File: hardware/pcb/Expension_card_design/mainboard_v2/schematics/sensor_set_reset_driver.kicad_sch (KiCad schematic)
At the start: 9 parts, among them U3 OPA2197xD

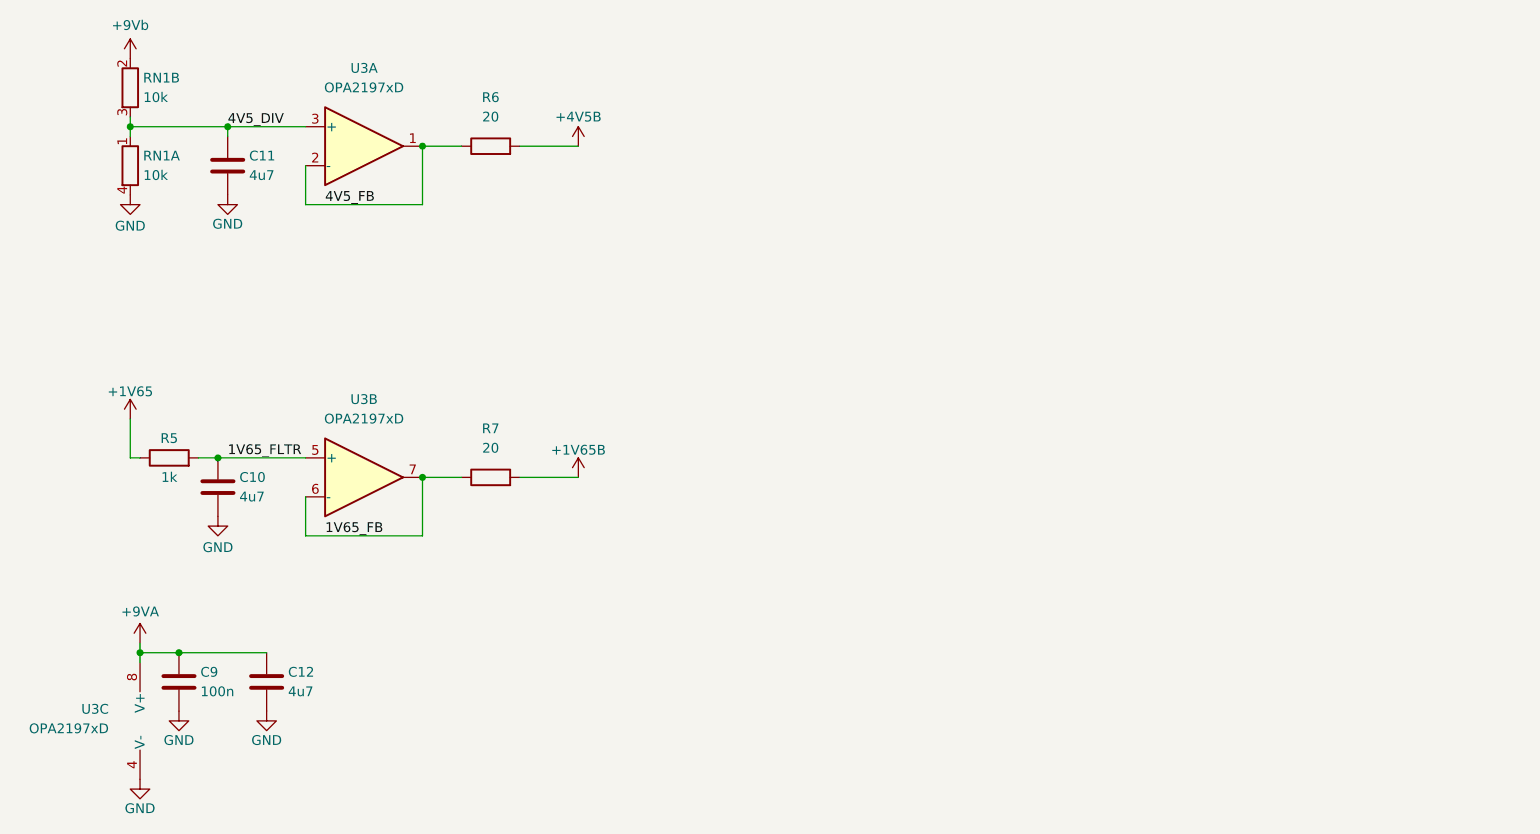
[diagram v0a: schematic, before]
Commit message: kicad mag board done
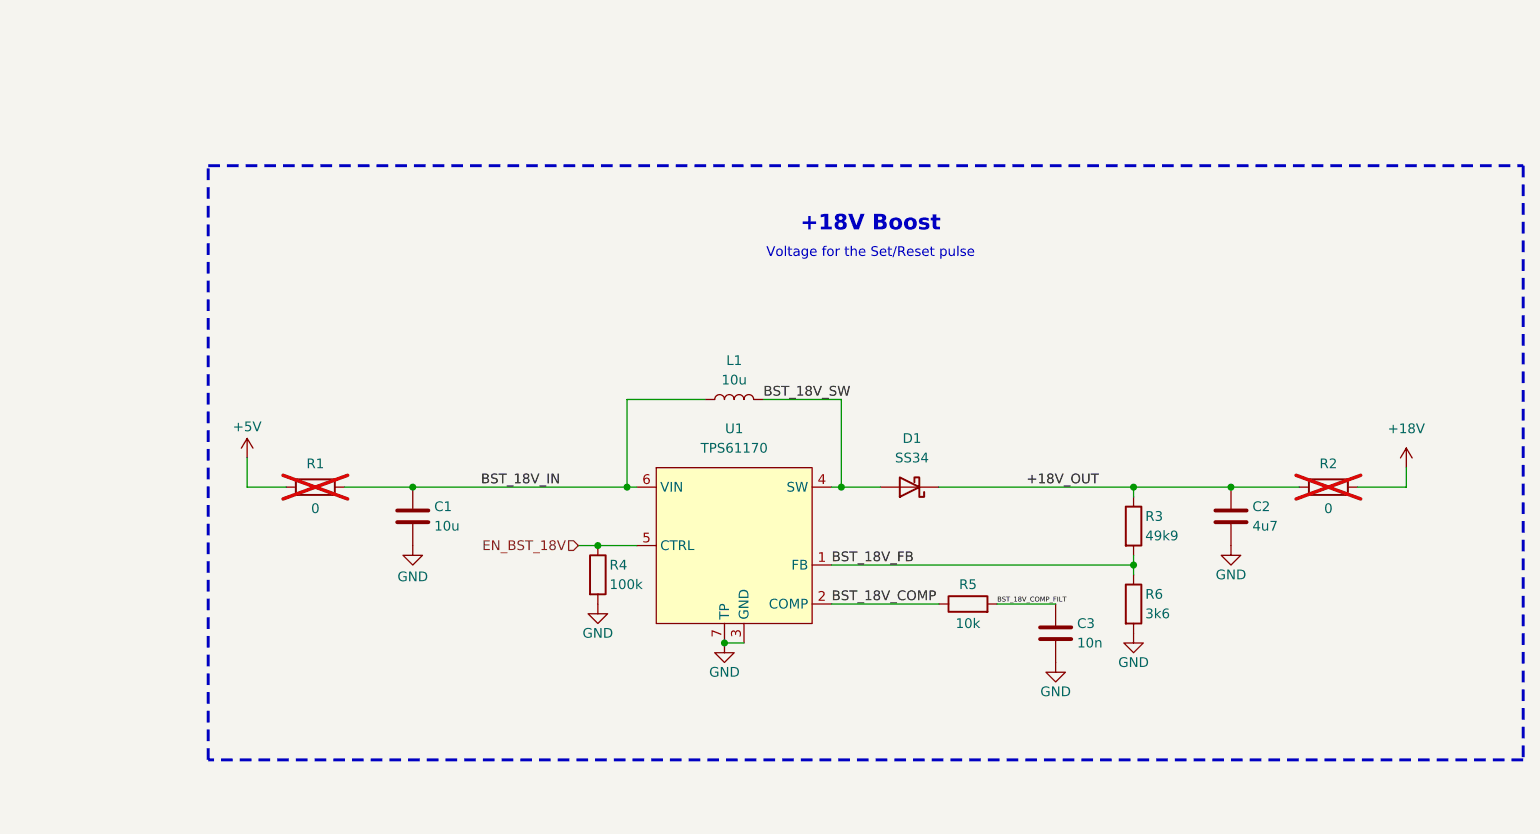
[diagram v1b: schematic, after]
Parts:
- removed C10, C11, C12: 4u7, Capacitor_SMD:C_1206_3216Metric, symbol Device:C
- removed C9: 100n, Capacitor_SMD:C_0603_1608Metric, symbol Device:C
- removed R7: 20, Resistor_SMD:R_0603_1608Metric, symbol Device:R
- removed RN1: 10k, Resistor_SMD:R_Array_Convex_2x0603, symbol Device:R_Pack02_Split
- removed U3: OPA2197xD, Package_SO:SOIC-8_3.9x4.9mm_P1.27mm, symbol Amplifier_Operational:OPA2197xD
- added C1: 10u, Capacitor_SMD:C_0805_2012Metric, symbol Device:C
- added C2: 4u7, Capacitor_SMD:C_1206_3216Metric, symbol Device:C
- added C3: 10n, Capacitor_SMD:C_0603_1608Metric, symbol Device:C
- added D1: SS34, Diode_SMD:D_SMA, symbol Device:D_Schottky
- added L1: 10u, magnode_footprints:ZEMS0850-100M_8.5x8.0mm, symbol Device:L
- added R1, R2: 0, Resistor_SMD:R_1206_3216Metric, symbol Device:R
- added R3: 49k9, Resistor_SMD:R_0603_1608Metric, symbol Device:R
- added R4: 100k, Resistor_SMD:R_0603_1608Metric, symbol Device:R
- added U1: TPS61170, Package_SON:WSON-6-1EP_2x2mm_P0.65mm_EP1x1.6mm, symbol magnode_symbols:TPS61170
- R5: value 1k -> 10k; LCSC C21190 -> C25804
- R6: value 20 -> 3k6; LCSC (none) -> C22980
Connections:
- net +4V5B is gone; now on net GND: R6.2
- net GND: now also C1.2, C2.2, C3.2, R4.2, U1.3 (GND), U1.7 (TP)
- net +1V65 renamed BST_18V_COMP
- net BST_18V_COMP: now also U1.2 (COMP)
- net 1V65_FLTR renamed BST_18V_COMP_FILT
- net BST_18V_COMP_FILT: now also C3.1
- net 4V5_FB renamed BST_18V_FB
- net BST_18V_FB: now also R3.2, U1.1 (FB)
- new net +18V: R2.2
- new net +18V_OUT: C2.1, D1.1 (K), R2.1, R3.1
- new net +5V: R1.1
- new net BST_18V_IN: C1.1, L1.1, R1.2, U1.6 (VIN)
- new net BST_18V_SW: D1.2 (A), L1.2, U1.4 (SW)
- new net EN_BST_18V: R4.1, U1.5 (CTRL)
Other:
- note added: "+18V Boost"
- note added: "Voltage for the Set/Reset pulse"
